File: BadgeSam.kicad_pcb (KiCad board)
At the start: 2 copper layers, 69.6 x 45 mm, 15 parts, among them SW1 RESET, U1 STM8S003F3P

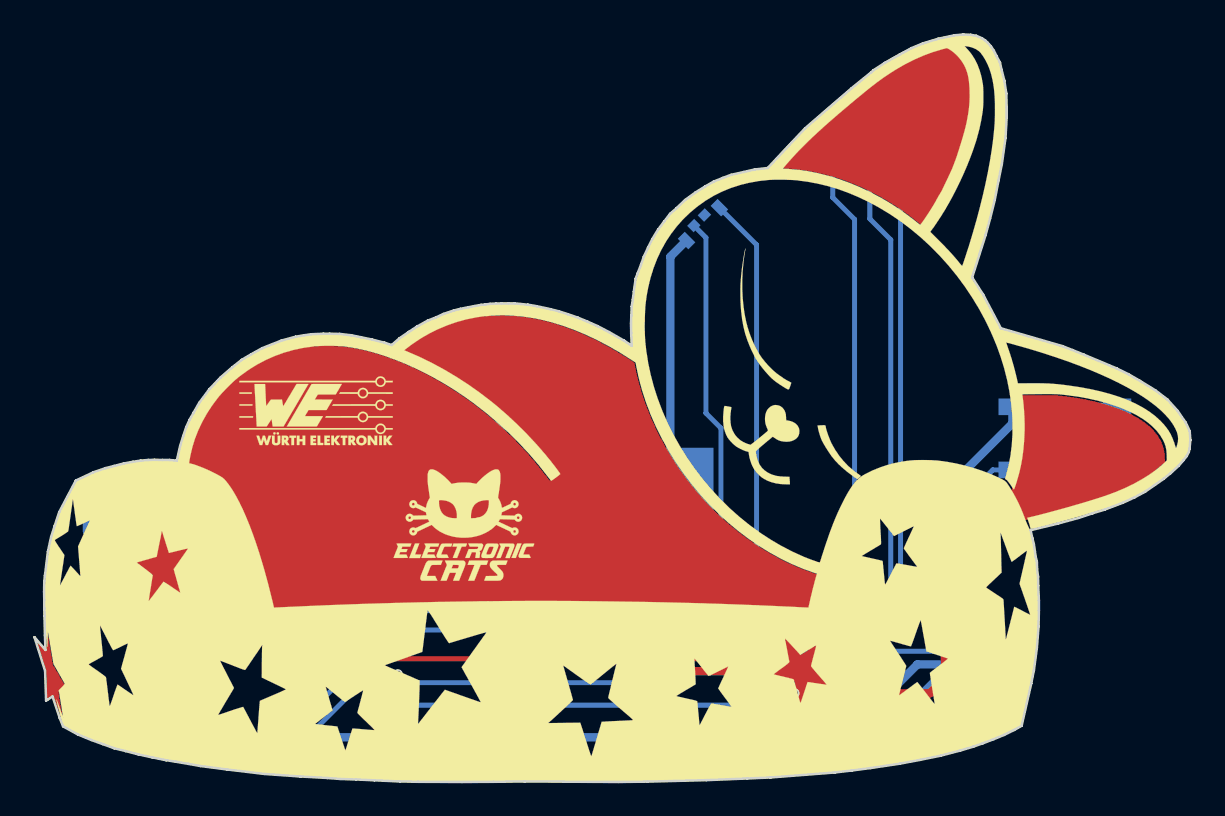
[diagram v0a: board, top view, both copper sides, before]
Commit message: fix routeo
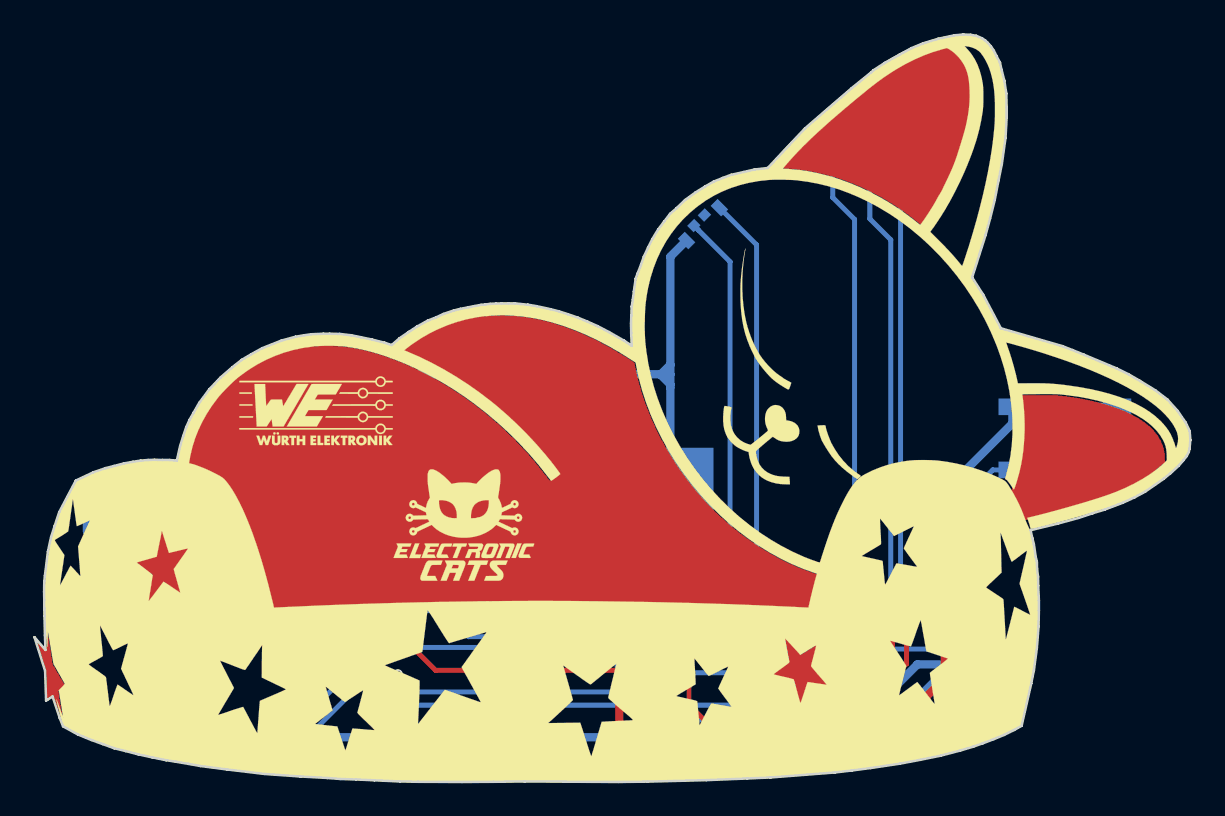
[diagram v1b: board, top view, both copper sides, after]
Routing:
- net /G1: track 49.0 -> 76.2 mm, vias 2 -> 3
- net /B1: track 48.5 -> 71.8 mm, vias 2 -> 4
- net +BATT: track 128.5 -> 137.4 mm, vias 4 -> 3
- net GND: track 85.9 -> 88.5 mm
- net Net-(C1-Pad1): track 10.3 -> 11.7 mm
- net /R1: track 54.7 -> 55.7 mm
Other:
- net class vcc: trace_width 0.3 -> 0.5
